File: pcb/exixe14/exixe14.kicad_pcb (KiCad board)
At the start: 2 copper layers, 47 parts, among them J1 Conn_01x07, J2 Conn_01x07, Q1 Q_PNP_BEC, Q10 Q_NPN_BEC, Q11 Q_NPN_BEC, Q12 Q_NPN_BEC, Q13 Q_NPN_BEC, Q14 Q_NPN_BEC, Q2 Q_NPN_BEC, Q3 Q_NPN_BEC, Q4 Q_NPN_BEC, Q5 Q_NPN_BEC, Q6 Q_NPN_BEC, Q7 Q_NPN_BEC, Q8 Q_NPN_BEC, Q9 Q_NPN_BEC, U1 STM32F042K6Tx

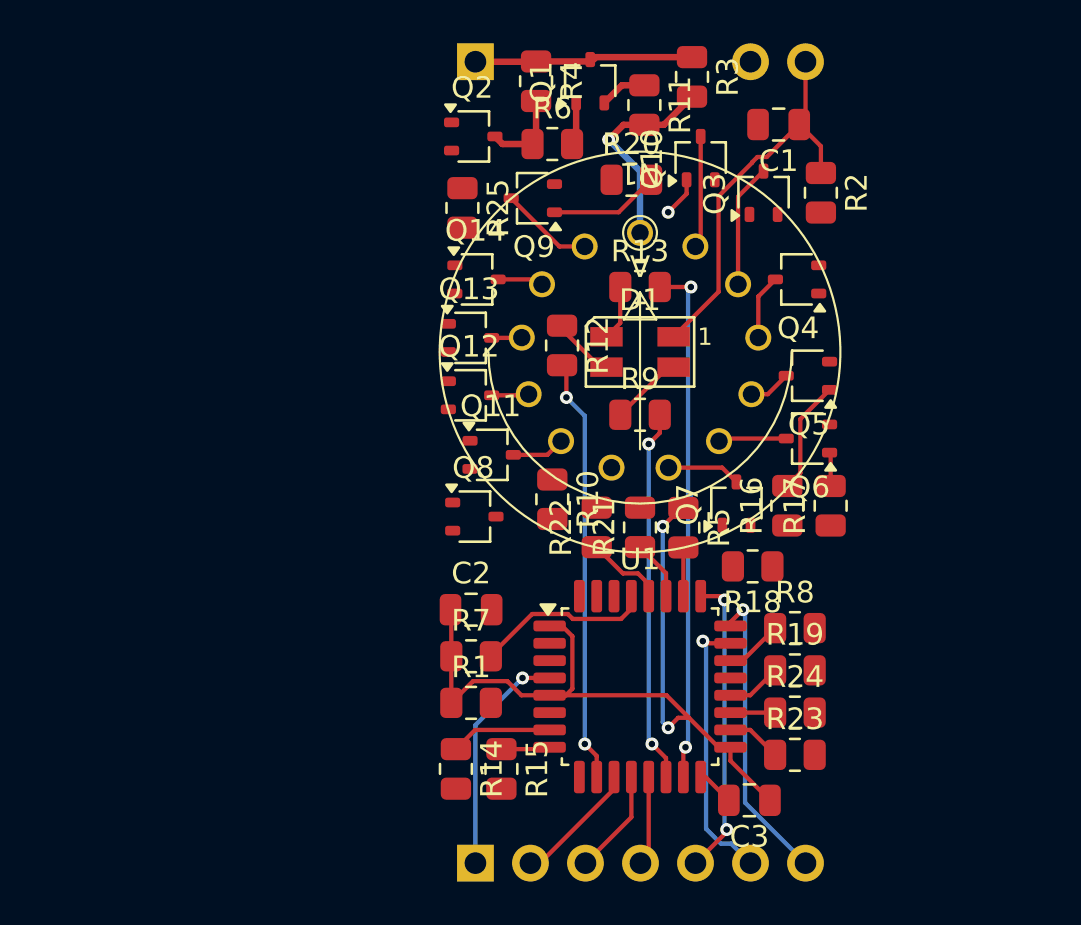
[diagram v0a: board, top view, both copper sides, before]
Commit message: pcb layout is hard
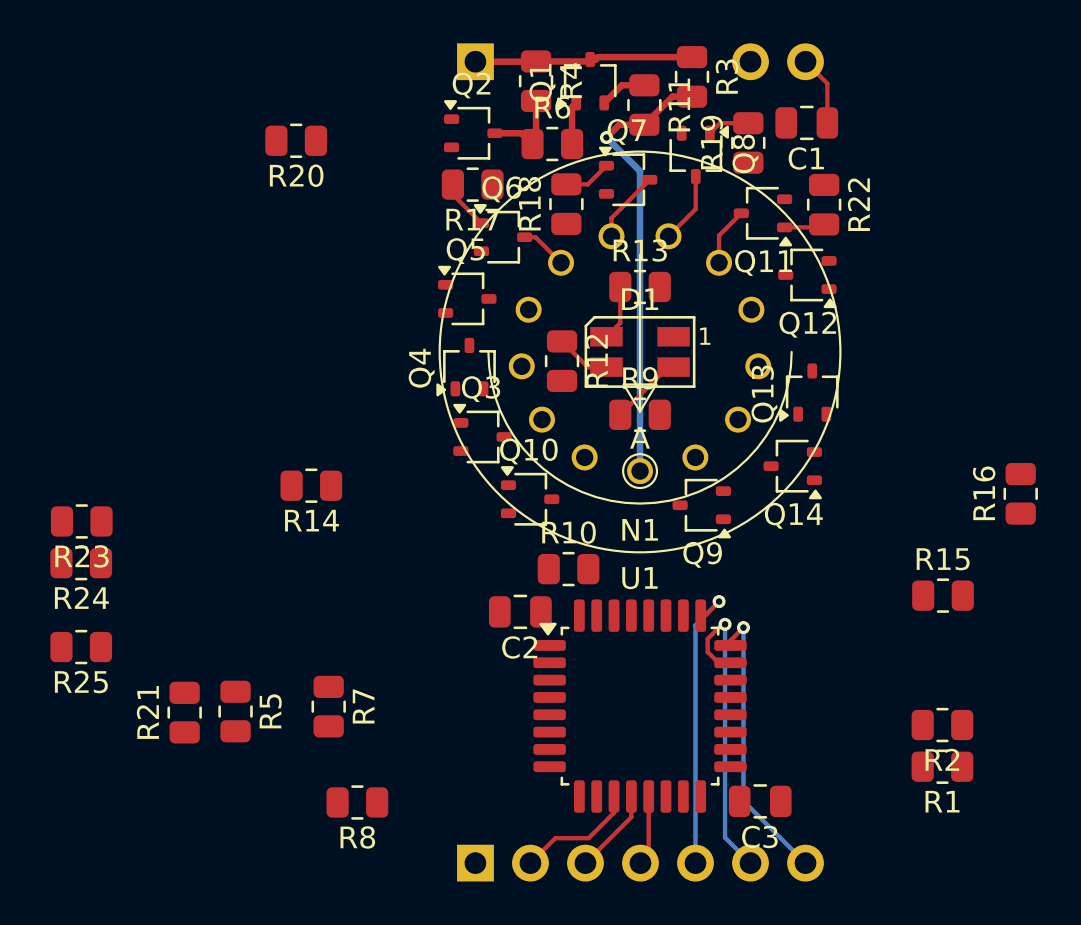
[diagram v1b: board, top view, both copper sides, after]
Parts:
- moved R23 34.6 mm to (34.2, 72.7), turned to 180 degrees
- moved R24 33.7 mm to (34.2, 74.7), turned to 180 degrees
- moved R25 26.8 mm to (34.2, 78.5), turned to 180 degrees
- moved R2 25.2 mm to (74.0, 82.1), turned to 180 degrees
- moved R19 24.4 mm to (65.0, 55.2), turned to 90 degrees
- moved R21 22.7 mm to (39.0, 81.5)
- moved R5 22.3 mm to (41.3, 81.5)
- moved R17 22.2 mm to (52.3, 57.2), turned to 180 degrees
- moved R1 22.0 mm to (74.0, 84.0), turned to 180 degrees
- moved R15 21.9 mm to (74.0, 76.2), turned to 0 degrees
- moved R8 21.7 mm to (47.0, 85.7), turned to 180 degrees
- moved Q8 19.6 mm to (62.6, 55.8), turned to -90 degrees
- moved R18 18.8 mm to (56.6, 58.1), turned to 90 degrees
- moved R22 18.2 mm to (68.5, 58.1), turned to -90 degrees
- moved Q10 17.6 mm to (54.9, 71.7), turned to 0 degrees
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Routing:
- net +3.3V: track 56.9 -> 3.24 mm, vias 2 -> 0
- net /PWM_RED: track 24.8 -> 0.00 mm, vias 2 -> 0
- net /PWM_GREEN: track 19.7 -> 0.00 mm, vias 2 -> 0
- net /PWM_BLUE: track 17.3 -> 0.00 mm, vias 2 -> 0
- net HV: track 9.57 -> 20.8 mm
- net /NRST: track 10.7 -> 0.00 mm, vias 1 -> 0
- net Net-(U1-PB6): track 8.19 -> 0.00 mm
- net /NIXIE_1: track 5.71 -> 0.00 mm
- net Net-(Q5-B): track 5.25 -> 0.00 mm
- net /NIXIE_LEFT: track 5.18 -> 0.00 mm
- net Net-(Q9-B): track 5.08 -> 0.00 mm
- net /STM_1: track 4.69 -> 0.00 mm
- net /NIXIE_RIGHT: track 4.32 -> 0.00 mm
- net /STM_7: track 3.66 -> 0.00 mm
- net /NIXIE_2: track 3.01 -> 0.00 mm
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
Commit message: working on exixe14 pcb
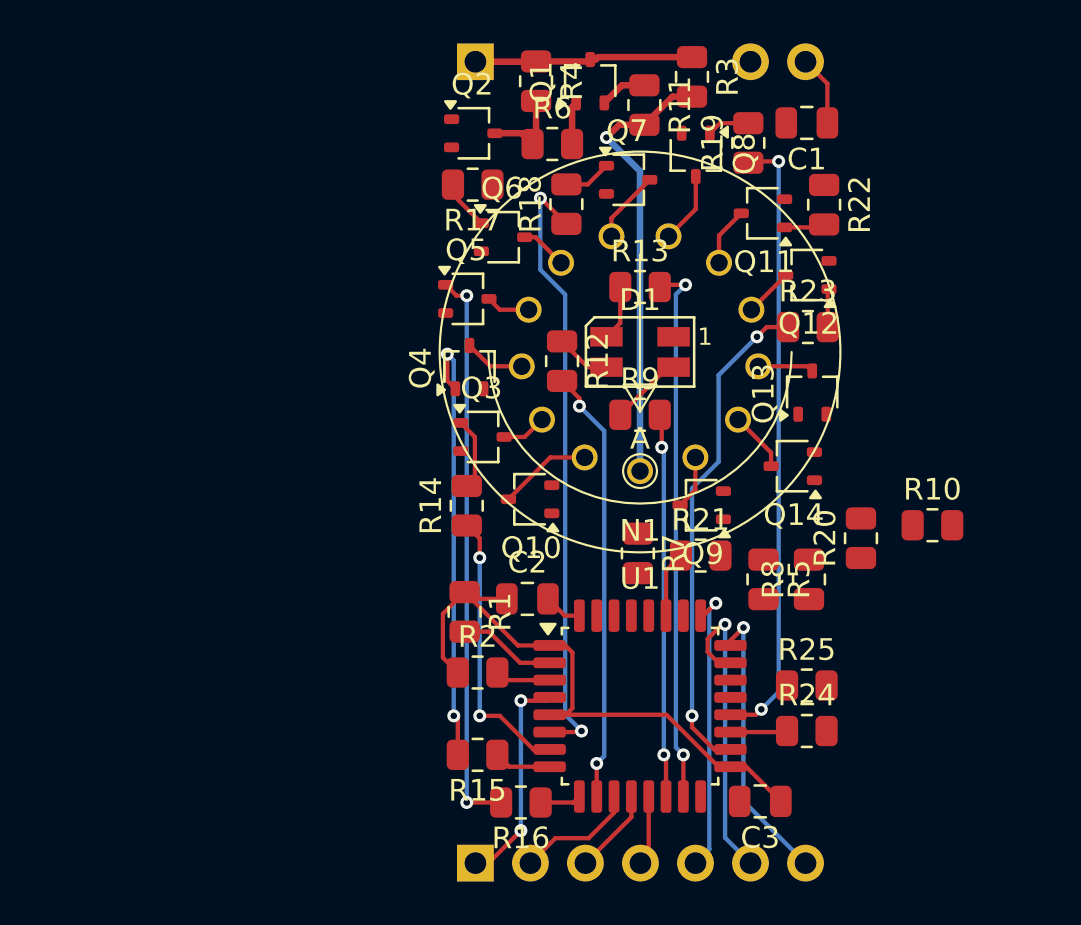
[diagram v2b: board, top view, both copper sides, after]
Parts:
- moved R23 34.7 mm to (67.8, 63.8), turned to 0 degrees
- moved R24 34.4 mm to (67.7, 82.4), turned to 0 degrees
- moved R25 33.5 mm to (67.7, 80.3), turned to 0 degrees
- moved R20 31.9 mm to (70.2, 73.5), turned to 90 degrees
- moved R16 27.1 mm to (54.5, 85.7), turned to 180 degrees
- moved R5 25.1 mm to (65.7, 75.4)
- moved R21 24.9 mm to (62.8, 74.3), turned to 0 degrees
- moved R8 23.3 mm to (67.8, 75.4), turned to 90 degrees
- moved R1 23.2 mm to (51.9, 76.9), turned to -90 degrees
- moved R15 22.7 mm to (52.5, 83.5), turned to 180 degrees
- moved R2 21.6 mm to (52.5, 79.7), turned to 0 degrees
- moved R10 16.9 mm to (73.5, 72.9)
- moved R7 15.9 mm to (59.9, 74.2)
- moved R14 7.23 mm to (52.0, 72.0), turned to 90 degrees
- moved C2 0.68 mm to (54.8, 76.3), turned to 0 degrees
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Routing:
- net +3.3V: track 3.24 -> 31.9 mm
- net /STM_6: track 0.00 -> 28.6 mm, vias 0 -> 2
- net /STM_5: track 0.00 -> 28.6 mm, vias 0 -> 2
- net Net-(Q5-B): track 0.00 -> 26.2 mm, vias 0 -> 2
- net /PWM_RED: track 0.00 -> 25.2 mm, vias 0 -> 2
- net /STM_8: track 0.00 -> 23.1 mm, vias 0 -> 2
- net Net-(Q4-B): track 0.00 -> 20.5 mm, vias 0 -> 2
- net /PWM_GREEN: track 0.00 -> 20.1 mm, vias 0 -> 2
- net /PWM_BLUE: track 0.00 -> 17.7 mm, vias 0 -> 2
- net /STM_1: track 0.00 -> 12.9 mm, vias 0 -> 2
- net /NRST: track 0.00 -> 10.1 mm, vias 0 -> 2
- net /NIXIE_LEFT: track 0.00 -> 4.73 mm
- net Net-(U1-PF0): track 0.00 -> 4.52 mm
- net Net-(Q3-B): track 0.00 -> 3.34 mm
- net /STM_LEFT: track 0.00 -> 3.06 mm
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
